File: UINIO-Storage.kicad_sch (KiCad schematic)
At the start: 36 parts, among them J1 Conn_01x04_Pin, J2 Conn_01x04_Pin, J3 Conn_01x06_Pin, J4 Conn_01x08_Pin, J5 Conn_01x06_Pin, U1 I2C-24-EEPROM-SOIC8, U2 I2C-24-EEPROM-TSSOP8, U3 SPI-25-Flash-SOIC8, U4 ME6211, U5 SPI-25-Flash-WSON8

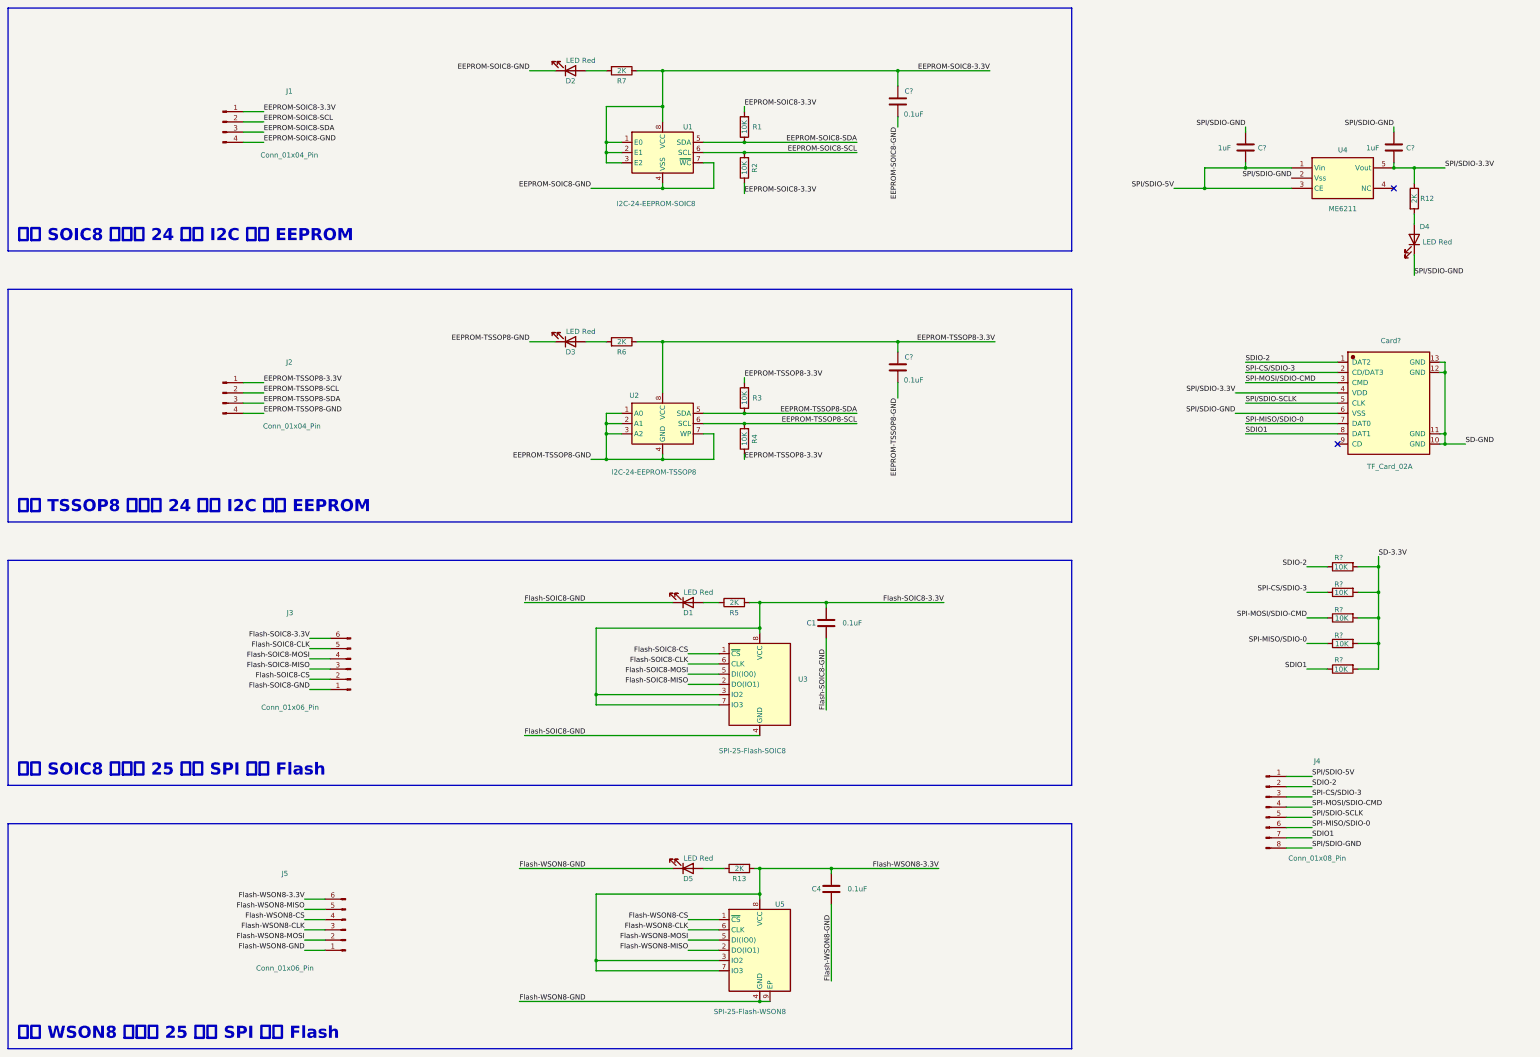
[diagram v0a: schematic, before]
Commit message: Finish PCB Layout.
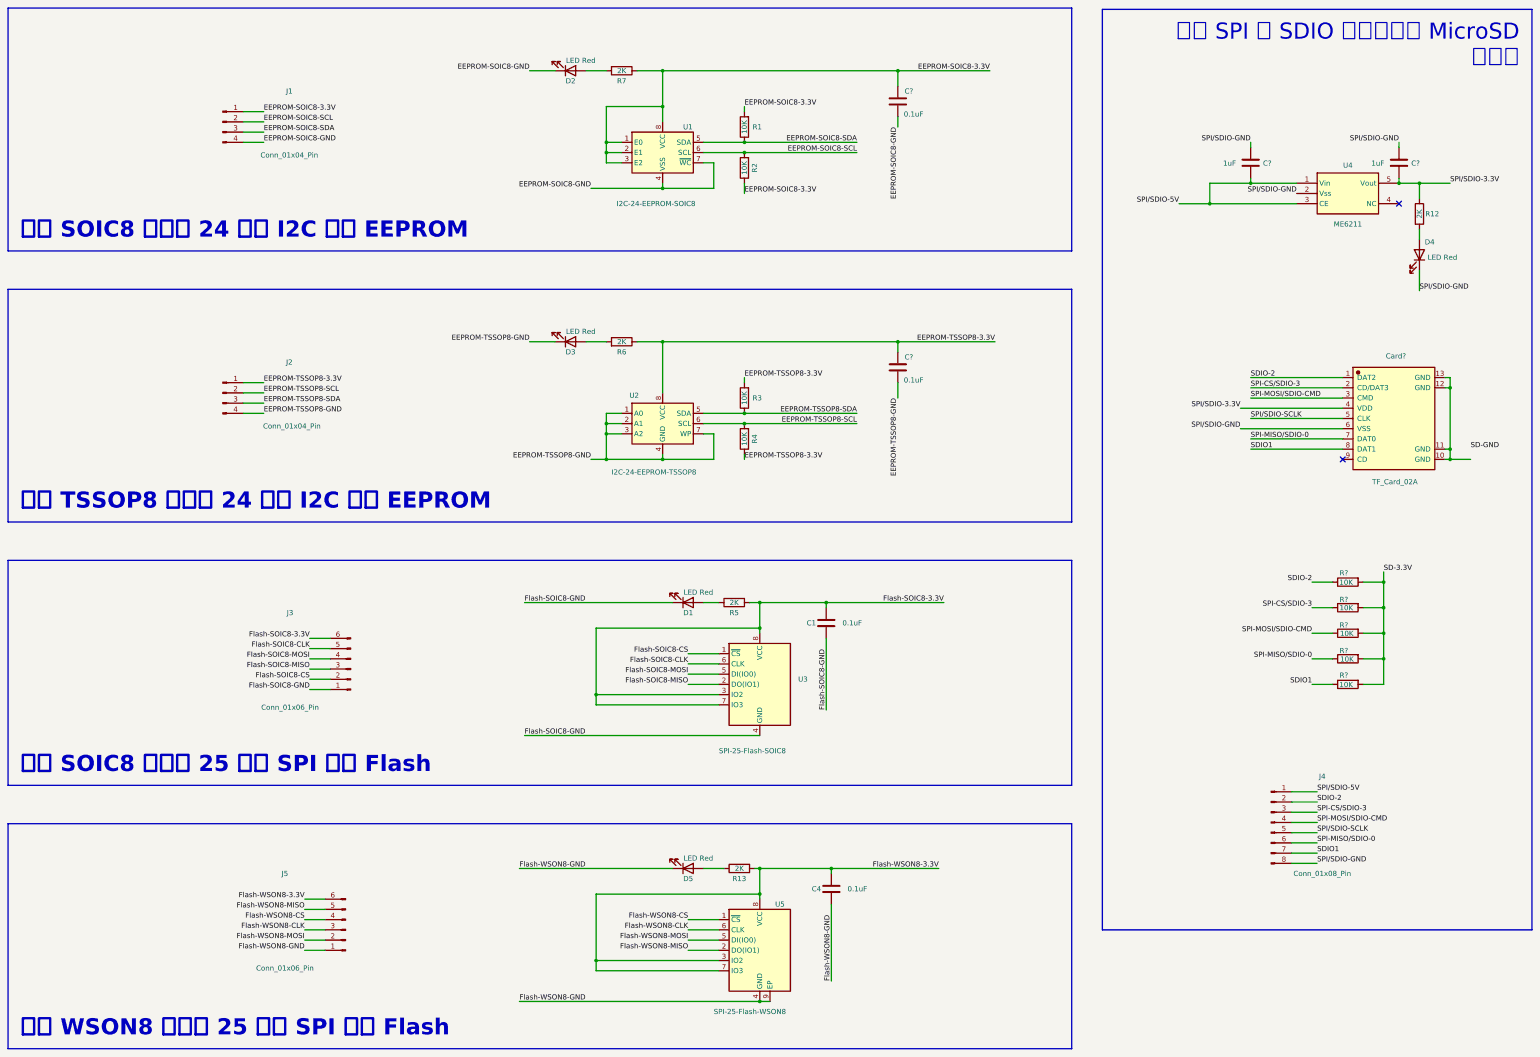
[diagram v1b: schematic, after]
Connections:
- net SD-GND: no longer Card?.10 (GND), Card?.11 (GND), Card?.12 (GND), Card?.13 (GND)
- new net: Card?.10 (GND), Card?.11 (GND), Card?.12 (GND), Card?.13 (GND)
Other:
- moved on the sheet: C?, Card?, D4, J4, R12, R?, U4
